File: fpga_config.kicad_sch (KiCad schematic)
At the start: 12 parts, among them J2 Molex 0878321420, U2 XC7A50T-FGG484

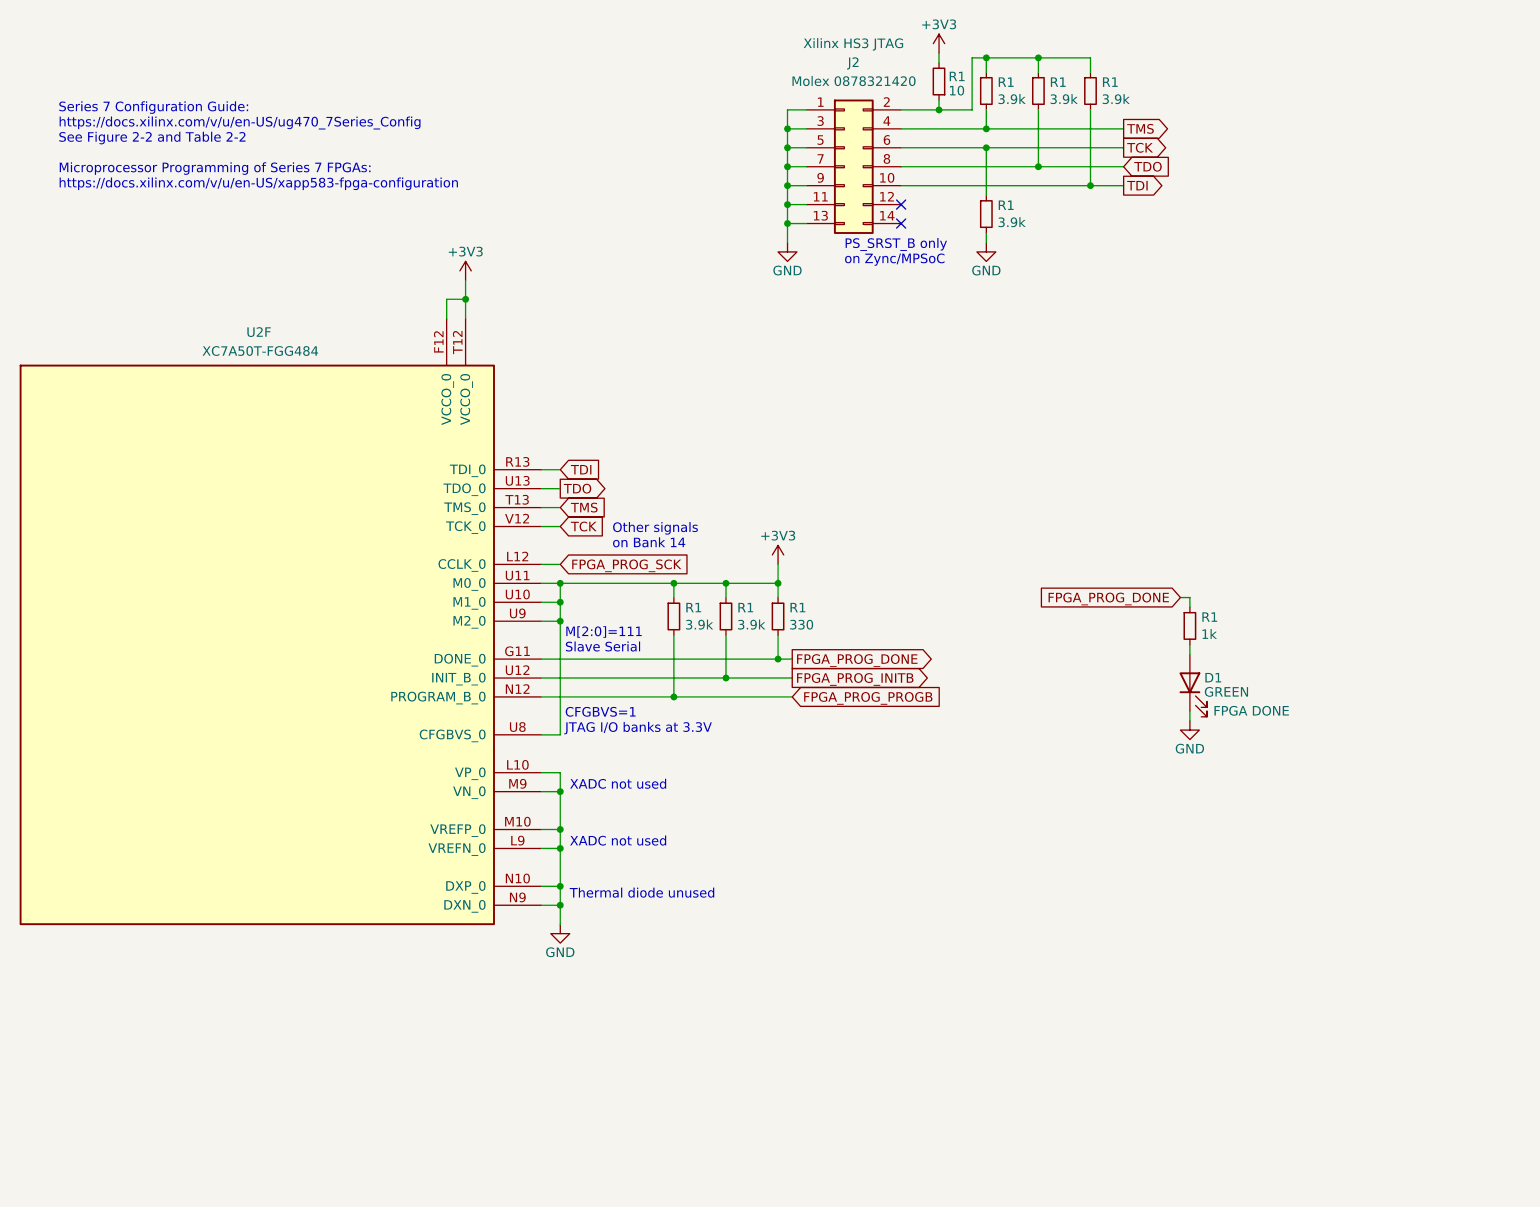
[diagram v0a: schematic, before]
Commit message: Schematic finished, starting layout
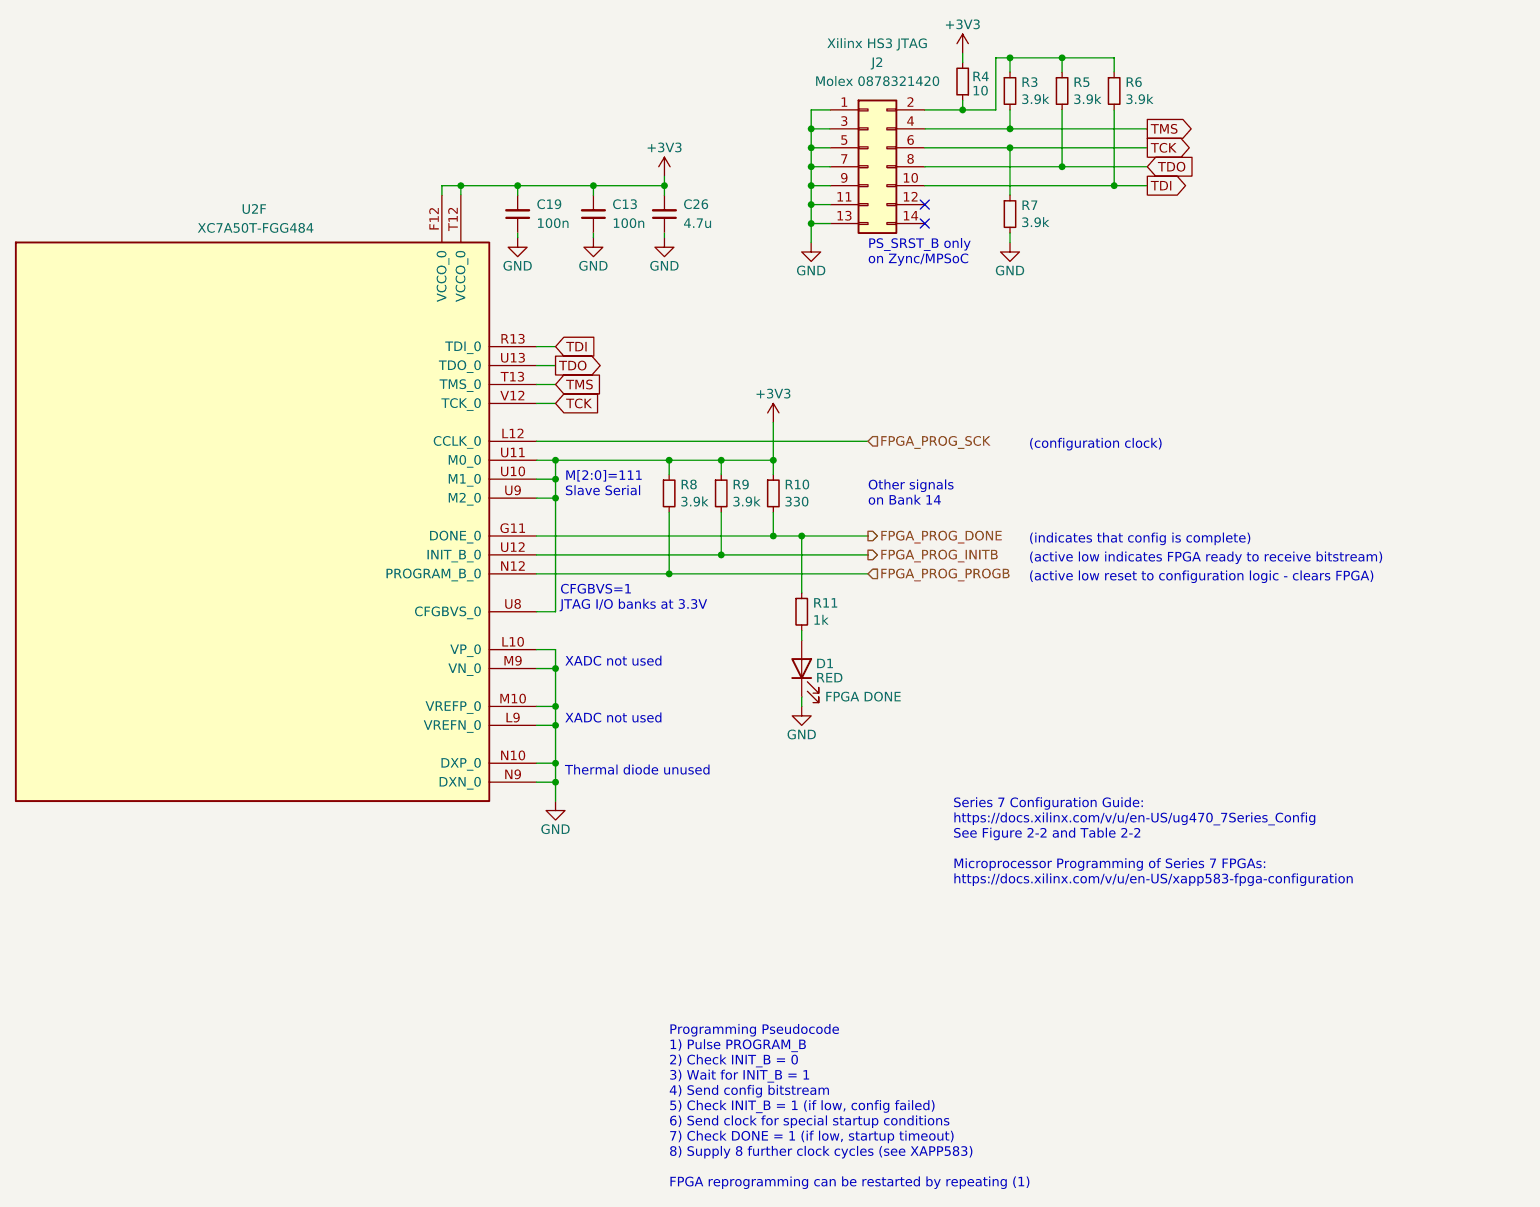
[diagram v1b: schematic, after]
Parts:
- added C13, C19: 100n, Capacitor_SMD:C_0402_1005Metric_Pad0.74x0.62mm_HandSolder, symbol Device:C_Small
- added C26: 4.7u, Capacitor_SMD:C_0402_1005Metric_Pad0.74x0.62mm_HandSolder, symbol Device:C_Small
- D1: value GREEN -> RED; footprint (none) -> LED_SMD:LED_0603_1608Metric_Pad1.05x0.95mm_HandSolder; LCSC (none) -> C2286
- R10: renamed from R1; footprint Resistor_SMD:R_0603_1608Metric_Pad0.98x0.95mm_HandSolder -> Resistor_SMD:R_0402_1005Metric_Pad0.72x0.64mm_HandSolder; LCSC C23138 -> (none)
- R11: renamed from R1; footprint Resistor_SMD:R_0603_1608Metric_Pad0.98x0.95mm_HandSolder -> Resistor_SMD:R_0402_1005Metric_Pad0.72x0.64mm_HandSolder; LCSC C21190 -> (none)
- R3, R5, R6, R7, R8, R9: renamed from R1; footprint Resistor_SMD:R_0603_1608Metric_Pad0.98x0.95mm_HandSolder -> Resistor_SMD:R_0402_1005Metric_Pad0.72x0.64mm_HandSolder; LCSC C23018 -> (none)
- R4: renamed from R1; footprint Resistor_SMD:R_0603_1608Metric_Pad0.98x0.95mm_HandSolder -> Resistor_SMD:R_0402_1005Metric_Pad0.72x0.64mm_HandSolder; LCSC C22859 -> (none)
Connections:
- net +3V3: now also C13.2, C19.2, C26.2
- net GND: now also C13.1, C19.1, C26.1
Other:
- note added: "(active low indicates FPGA ready to receive bitstream)"
- note added: "(active low reset to configuration logic - clears FPGA)"
- note added: "(configuration clock)"
- note added: "(indicates that config is complete)"
- note added: "Programming Pseudocode 1) Pulse PROGRAM_B 2) Check INIT_B = 0 3) Wait for INIT_B = 1 4) Send config bitstream 5) Check INIT_B = 1 (if low, config failed) 6) Send clock for special startup conditions 7) Check DONE = 1 (if low, startup timeout) 8) Supply 8 further clock cycles (see XAPP583) FPGA reprogramming can be restarted by repeating (1)"
- title: FPGA Configuration (Bank 0) -> FPGA Power
- moved on the sheet: D1, J2, R10, R11, R3, R4, R5, R6, R7, R8, R9, U2F
